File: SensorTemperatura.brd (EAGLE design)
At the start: 160 x 100 mm, 16 parts, among them IC1 MAX481CPA, IC2 MEGA8-P, Q1 16mhz

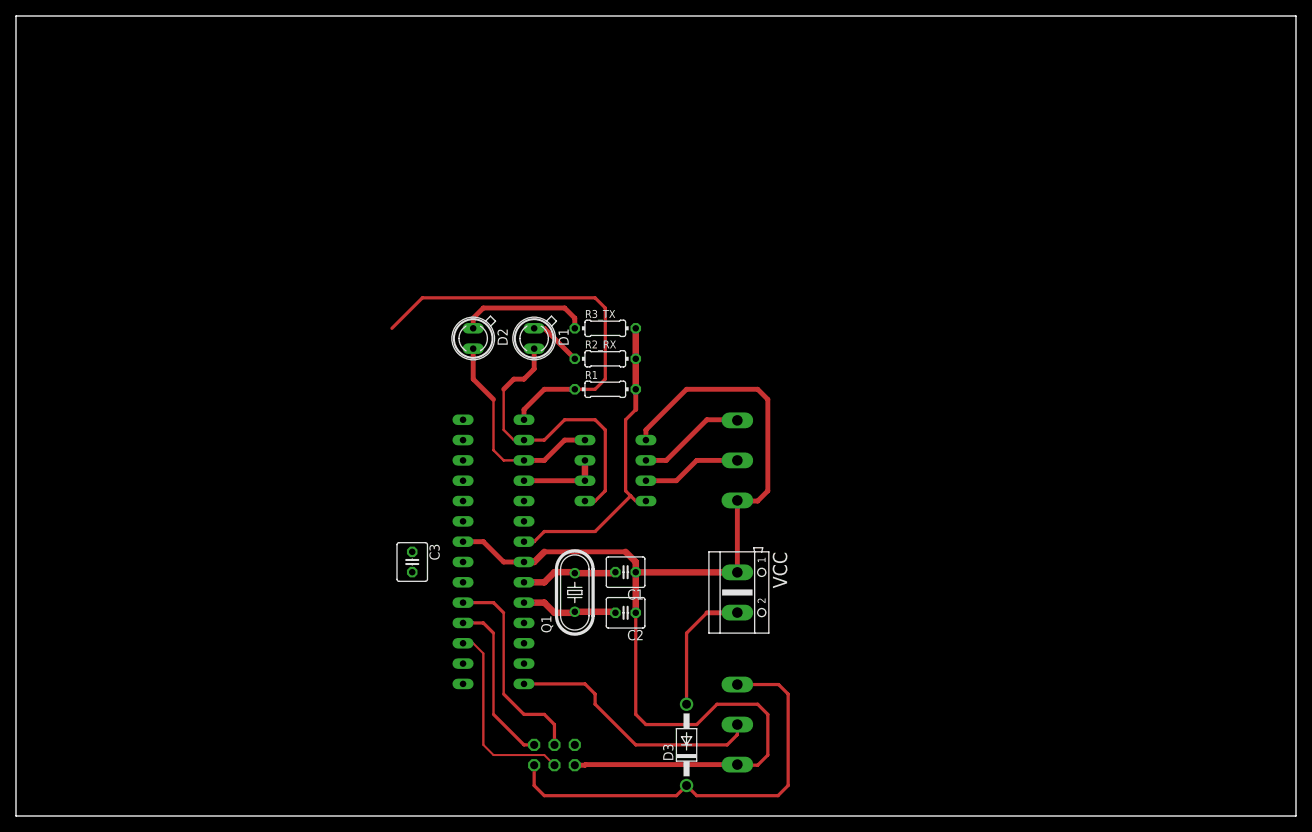
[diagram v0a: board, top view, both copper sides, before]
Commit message: fix terrena
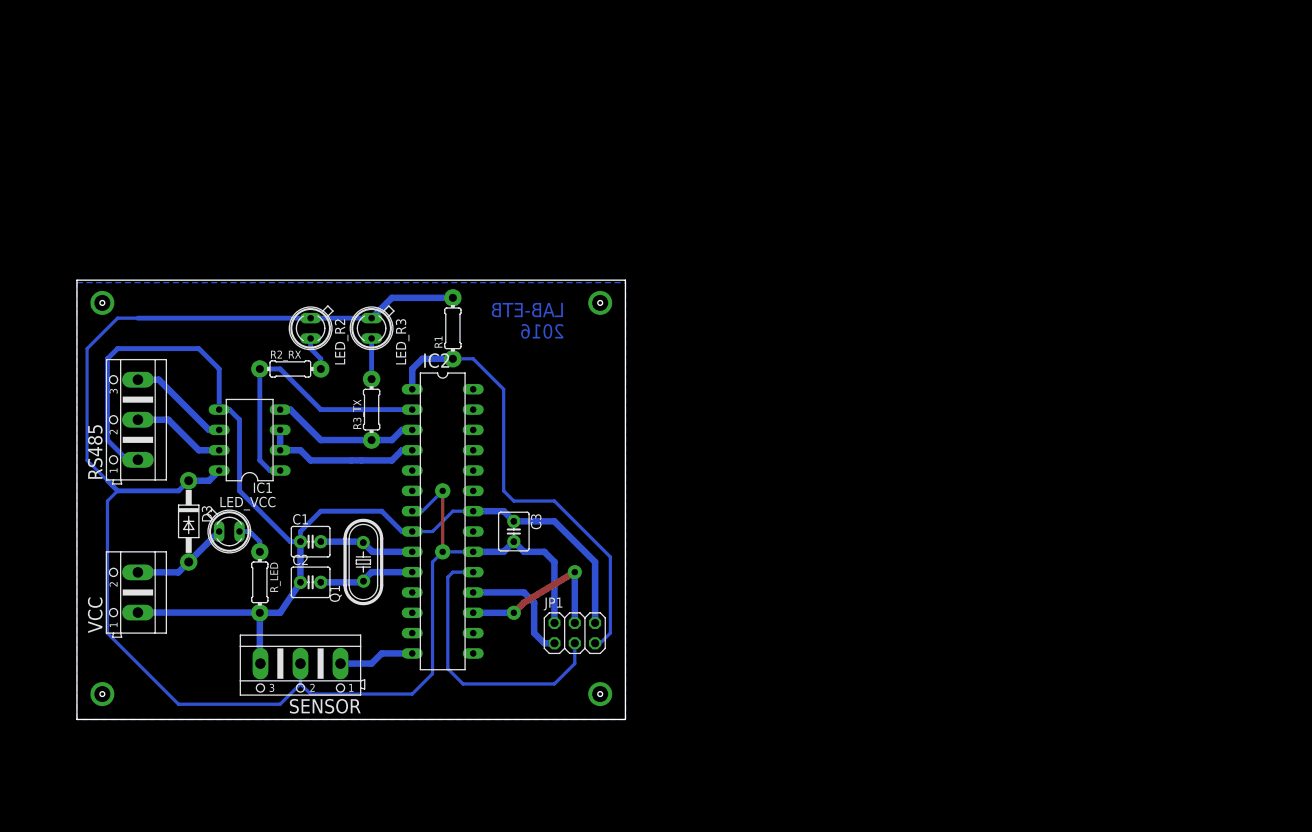
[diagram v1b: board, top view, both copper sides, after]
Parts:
- removed D1, D2: SFH482, led:SFH482
- added LED_R2, LED_R3: (no value), led:SFH482
- added LED_VCC: SFH482, led:SFH482
- added R_LED: (no value), rcl:0204/7
- moved RS485 75.1 mm to (15.2, 49.5), flipped to the top
- moved VCC 74.9 mm to (15.2, 27.9), turned to 90 degrees
- moved D3 68.2 mm to (21.6, 36.8), turned to 270 degrees
- moved SENSOR 55.1 mm to (35.6, 19.1), flipped to the top, turned to 180 degrees
- moved IC1 45.9 mm to (29.2, 47.0), flipped to the top
- moved C1 39.6 mm to (36.8, 34.3), turned to 0 degrees
- moved C2 39.6 mm to (36.8, 29.2), turned to 0 degrees
- moved R2_RX 39.4 mm to (34.3, 55.9)
- moved R3_TX 30.9 mm to (44.5, 50.8), turned to 90 degrees
- moved Q1 26.7 mm to (43.4, 31.8)
- moved R1 20.5 mm to (54.6, 61.0), turned to 90 degrees
- moved JP1 15.5 mm to (69.8, 22.9), flipped to the top, turned to 0 degrees
- moved C3 13.3 mm to (62.2, 35.6)
- moved IC2 7.41 mm to (53.3, 36.8), flipped to the top
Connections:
- new net N$17: LED_VCC.K, R_LED.1
- net GND: now also R_LED.2, SENSOR.3; no longer RS485.1, SENSOR.1
- net N$10: now also SENSOR.1; no longer SENSOR.2
- net N$15: now also LED_VCC.A
- net N$3: now also R2_RX.1; no longer D1.K
- net N$4: now also LED_R2.K, R2_RX.2; no longer D1.A, R2_RX.1
- net N$5: now also LED_R3.K, R3_TX.2; no longer D2.A, R3_TX.1
- net N$6: now also R3_TX.1; no longer D2.K
- net VCC: now also LED_R2.A, LED_R3.A, SENSOR.2; no longer R2_RX.2, R3_TX.2, SENSOR.3
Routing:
- net VCC: track 104.4 -> 200.7 mm, vias 0 -> 2
- net N$10: track 32.4 -> 9.49 mm
- net N$5: track 16.3 -> 5.08 mm
- net N$1: track 10.2 -> 20.1 mm
- net N$9: track 26.2 -> 35.1 mm
- net N$6: track 26.8 -> 18.6 mm
- net N$13: track 50.7 -> 57.5 mm
- net N$2: track 21.2 -> 15.0 mm
- net GND: track 147.8 -> 143.2 mm
- net N$17: track 0.00 -> 4.34 mm
- net N$15: track 16.3 -> 12.3 mm
- net N$14: track 24.4 -> 20.6 mm, vias 0 -> 2
- net N$4: track 6.66 -> 4.34 mm
- net N$3: track 38.0 -> 35.7 mm
- net N$7: track 13.6 -> 12.8 mm
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- added copper zone on layer 16, net S$15
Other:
- board size 160 x 100 mm -> 68.6 x 54.9 mm
- board text added: "LAB-ETB 2016"

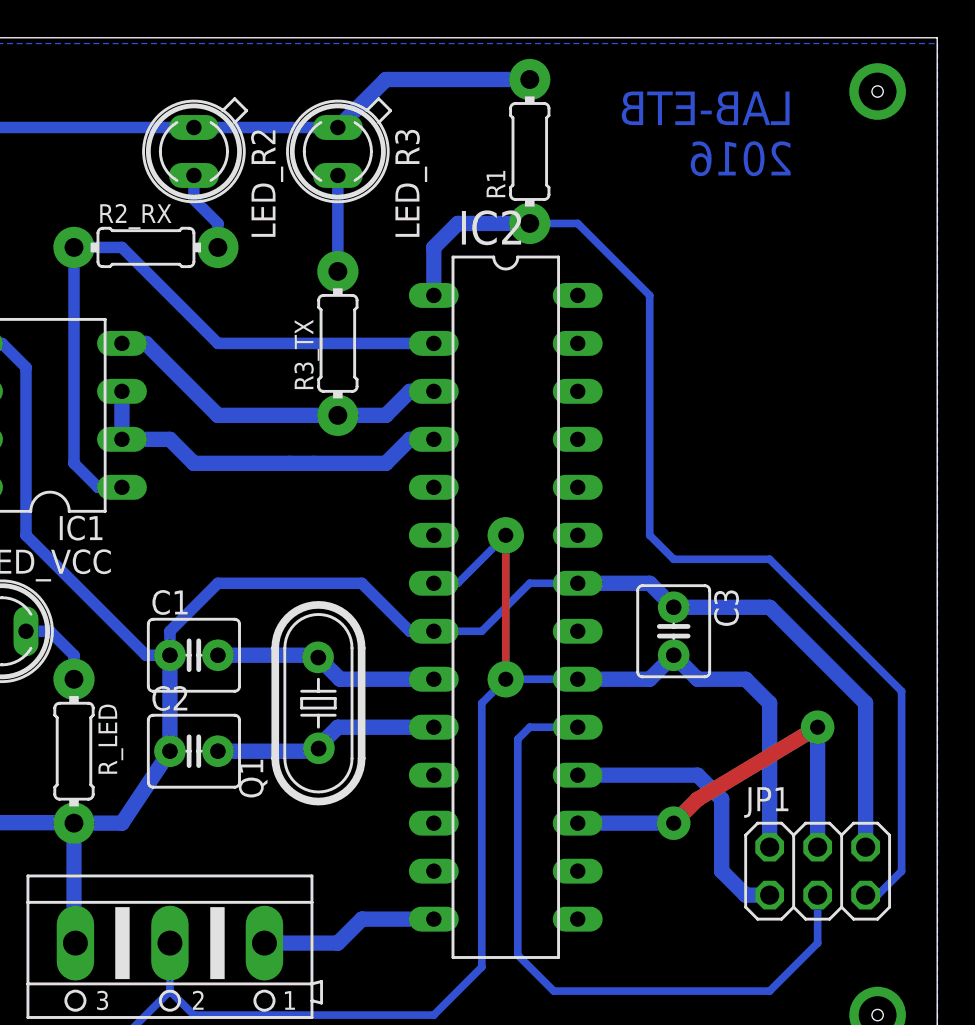
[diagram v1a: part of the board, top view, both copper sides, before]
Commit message: fix
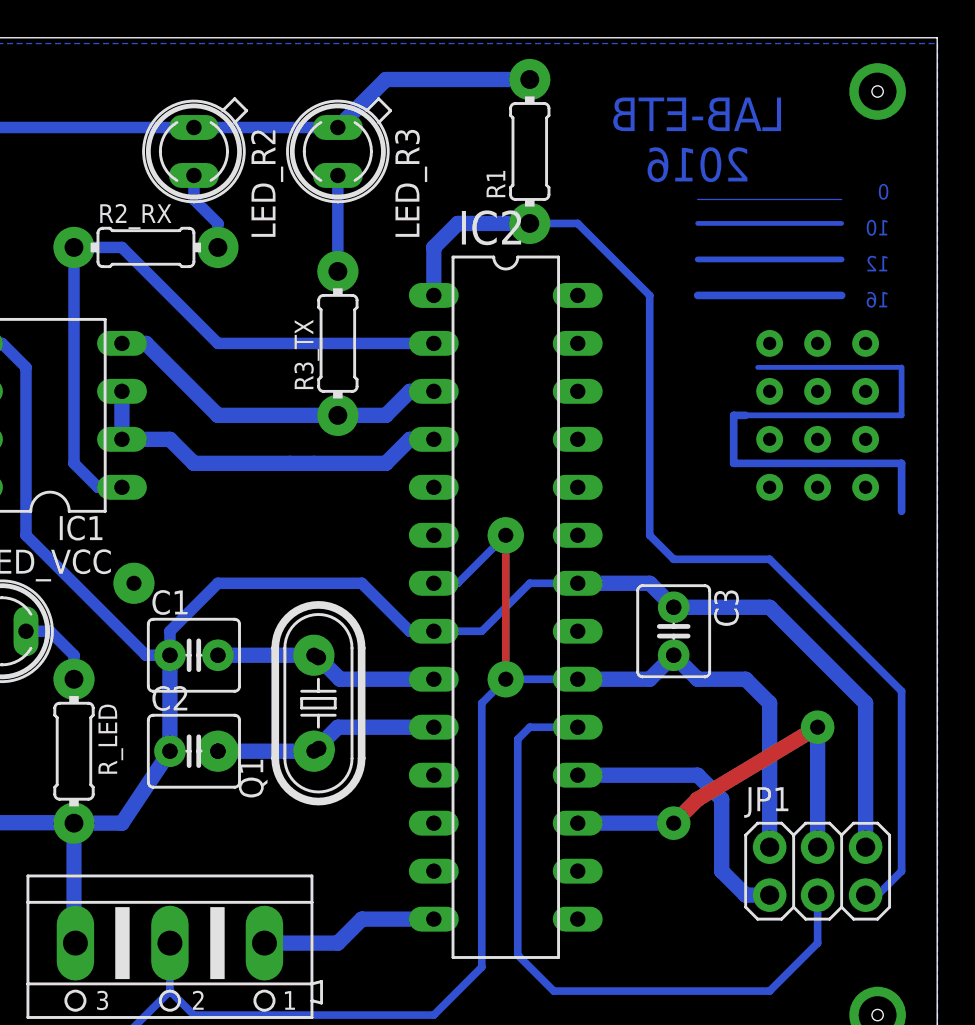
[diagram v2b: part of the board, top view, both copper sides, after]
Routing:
- net S$36: track 0.00 -> 33.0 mm
- net S$40: track 0.00 -> 7.62 mm
- net S$39: track 0.00 -> 7.62 mm
- net S$38: track 0.00 -> 7.62 mm
- net S$37: track 0.00 -> 7.62 mm
- added copper zone on layer 16, net GND
- removed copper zone on layer 16, net S$15
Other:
- board text added: "0"
- board text added: "10"
- board text added: "12"
- board text added: "16"
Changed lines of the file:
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@@
 <layer number="17" name="Pads" color="2" fill="1" visible="yes" active="yes"/>
 <layer number="18" name="Vias" color="2" fill="1" visible="yes" active="yes"/>
-<layer number="19" name="Unrouted" color="6" fill="1" visible="no" active="yes"/>
+<layer number="19" name="Unrouted" color="6" fill="1" visible="yes" active="yes"/>
 <layer number="20" name="Dimension" color="15" fill="1" visible="yes" active="yes"/>
 <layer number="21" name="tPlace" color="7" fill="1" visible="no" active="yes"/>
@@
 <wire x1="76.18" y1="66.98" x2="7.62" y2="66.98" width="0" layer="20"/>
 <wire x1="7.62" y1="66.98" x2="7.62" y2="12.065" width="0" layer="20"/>
-<text x="68.58" y="59.69" size="1.778" layer="16" rot="MR0">LAB-ETB
+<text x="63.5" y="61.595" size="1.778" layer="16" rot="MR0" align="center">LAB-ETB
 2016</text>
 <hole x="10.795" y="64.135" drill="0.6"/>
@@
 <hole x="73.025" y="15.24" drill="0.6"/>
 <hole x="10.795" y="15.24" drill="0.6"/>
+<text x="73.66" y="58.42" size="0.8128" layer="16" rot="MR0">0</text>
+<text x="73.66" y="56.515" size="0.8128" layer="16" rot="MR0">10</text>
+<text x="73.66" y="54.61" size="0.8128" layer="16" rot="MR0">12</text>
+<text x="73.66" y="52.705" size="0.8128" layer="16" rot="MR0">16</text>
 </plain>
 <attributes>
@@
 <wire x1="22.86" y1="58.42" x2="25.4" y2="55.88" width="0.6096" layer="16"/>
 <wire x1="25.4" y1="55.88" x2="25.4" y2="50.8" width="0.6096" layer="16"/>
+<polygon width="0.4064" layer="16" spacing="0.8128" isolate="1.27" orphans="yes">
+<vertex x="7.62" y="66.675"/>
+<vertex x="76.2" y="66.675"/>
+<vertex x="76.2" y="12.065"/>
+<vertex x="7.62" y="12.065"/>
+</polygon>
 </signal>
 <signal name="N$1">
@@
 </signal>
 <signal name="S$15">
-<polygon width="0.254" layer="16" spacing="0.6096" isolate="1.27" orphans="yes">
-<vertex x="7.62" y="66.675"/>
-<vertex x="76.2" y="66.675"/>
-<vertex x="76.2" y="12.065"/>
-<vertex x="7.62" y="12.065"/>
-</polygon>
+<via x="67.31" y="21.59" extent="1-16" drill="0.6" diameter="1.778"/>
+</signal>
+<signal name="S$16">
+<via x="72.39" y="24.13" extent="1-16" drill="0.6" diameter="1.778"/>
+</signal>
+<signal name="S$17">
+<via x="72.39" y="21.59" extent="1-16" drill="0.6" diameter="1.778"/>
+</signal>
+<signal name="S$18">
+<via x="69.85" y="24.13" extent="1-16" drill="0.6" diameter="1.778"/>
+</signal>
+<signal name="S$19">
+<via x="69.85" y="21.59" extent="1-16" drill="0.6" diameter="1.778"/>
+</signal>
+<signal name="S$20">
+<via x="67.31" y="24.13" extent="1-16" drill="0.6" diameter="1.778"/>
+</signal>
+<signal name="S$21">
+<via x="43.18" y="29.21" extent="1-16" drill="0.8" diameter="2.1844"/>
+</signal>
+<signal name="S$22">
+<via x="43.18" y="34.29" extent="1-16" drill="0.8" diameter="2.1844"/>
+</signal>
+<signal name="S$23">
+<via x="38.1" y="29.21" extent="1-16" drill="0.8" diameter="2.1844"/>
+</signal>
+<signal name="S$24">
+<via x="33.655" y="38.1" extent="1-16" drill="0.8" diameter="2.1844"/>
+</signal>
+<signal name="S$25">
+<via x="67.31" y="50.8" extent="1-16" drill="0.7" diameter="1.4224"/>
+</signal>
+<signal name="S$26">
+<via x="67.31" y="48.26" extent="1-16" drill="0.7" diameter="1.4224"/>
+</signal>
+<signal name="S$27">
+<via x="69.85" y="50.8" extent="1-16" drill="0.7" diameter="1.4224"/>
+</signal>
+<signal name="S$28">
+<via x="72.39" y="50.8" extent="1-16" drill="0.7" diameter="1.4224"/>
+</signal>
+<signal name="S$29">
+<via x="72.39" y="48.26" extent="1-16" drill="0.7" diameter="1.4224"/>
+</signal>
+<signal name="S$30">
+<via x="69.85" y="48.26" extent="1-16" drill="0.7" diameter="1.4224"/>
+<via x="67.31" y="45.72" extent="1-16" drill="0.7" diameter="1.4224"/>
+<wire x1="67.31" y1="45.72" x2="69.85" y2="48.26" width="0" layer="19" extent="1-1"/>
+</signal>
+<signal name="S$31">
+<via x="69.85" y="45.72" extent="1-16" drill="0.7" diameter="1.4224"/>
+</signal>
+<signal name="S$32">
+<via x="72.39" y="45.72" extent="1-16" drill="0.7" diameter="1.4224"/>
+</signal>
+<signal name="S$33">
+<via x="67.31" y="43.18" extent="1-16" drill="0.7" diameter="1.4224"/>
+</signal>
+<signal name="S$34">
+<via x="69.85" y="43.18" extent="1-16" drill="0.7" diameter="1.4224"/>
+</signal>
+<signal name="S$35">
+<via x="72.39" y="43.18" extent="1-16" drill="0.7" diameter="1.4224"/>
+</signal>
+<signal name="S$36">
+<wire x1="66.675" y1="49.53" x2="74.295" y2="49.53" width="0.254" layer="16"/>
+<wire x1="74.295" y1="49.53" x2="74.295" y2="46.99" width="0.3048" layer="16"/>
+<wire x1="74.295" y1="46.99" x2="66.04" y2="46.99" width="0.3048" layer="16"/>
+<wire x1="66.04" y1="46.99" x2="65.405" y2="46.99" width="0.4064" layer="16"/>
+<wire x1="65.405" y1="46.99" x2="65.405" y2="44.45" width="0.4064" layer="16"/>
+<wire x1="65.405" y1="44.45" x2="74.295" y2="44.45" width="0.4064" layer="16"/>
+<wire x1="74.295" y1="44.45" x2="74.295" y2="41.91" width="0.4064" layer="16"/>
+</signal>
+<signal name="S$37">
+<wire x1="63.5" y1="58.42" x2="71.12" y2="58.42" width="0" layer="16"/>
+</signal>
+<signal name="S$38">
+<wire x1="63.5" y1="57.15" x2="71.12" y2="57.15" width="0.254" layer="16"/>
+</signal>
+<signal name="S$39">
+<wire x1="63.5" y1="55.245" x2="71.12" y2="55.245" width="0.3048" layer="16"/>
+</signal>
+<signal name="S$40">
+<wire x1="63.5" y1="53.34" x2="71.12" y2="53.34" width="0.4064" layer="16"/>
 </signal>
 </signals>
